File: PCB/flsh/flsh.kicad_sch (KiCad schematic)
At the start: 10 parts, among them U1 0.18Ω, U2 0.18Ω, U3 0.18Ω, U4 0.18Ω, U5 0.18Ω

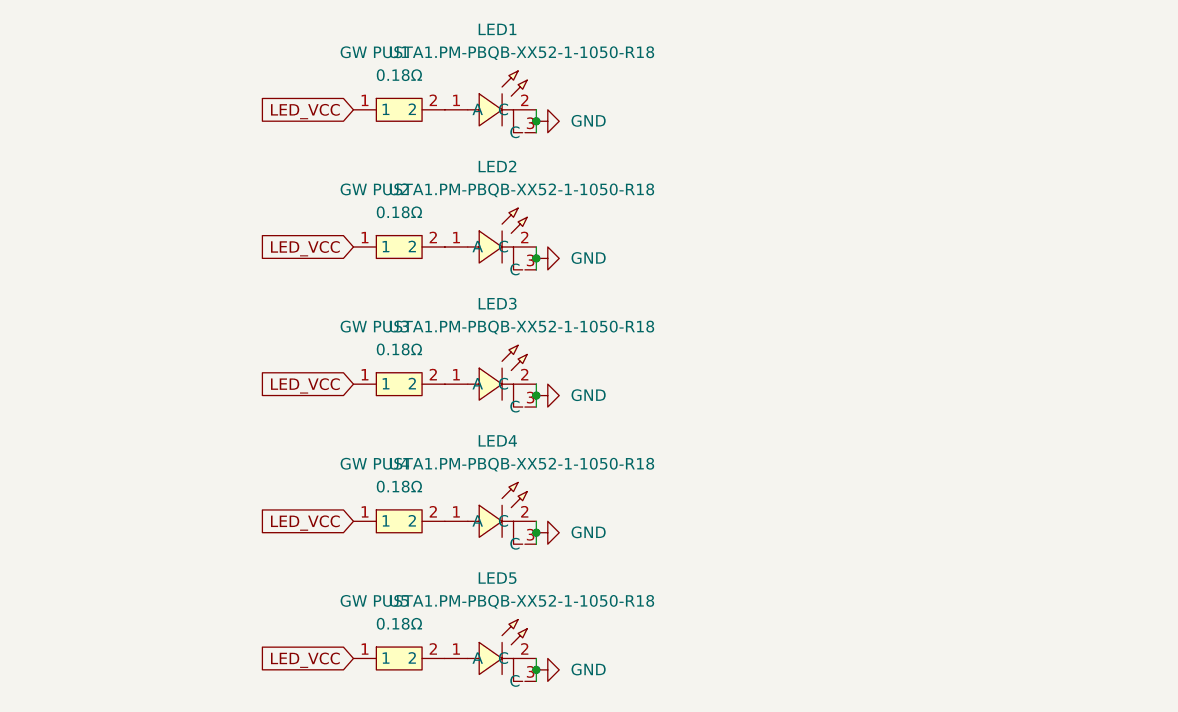
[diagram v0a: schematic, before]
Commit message: flsh!!
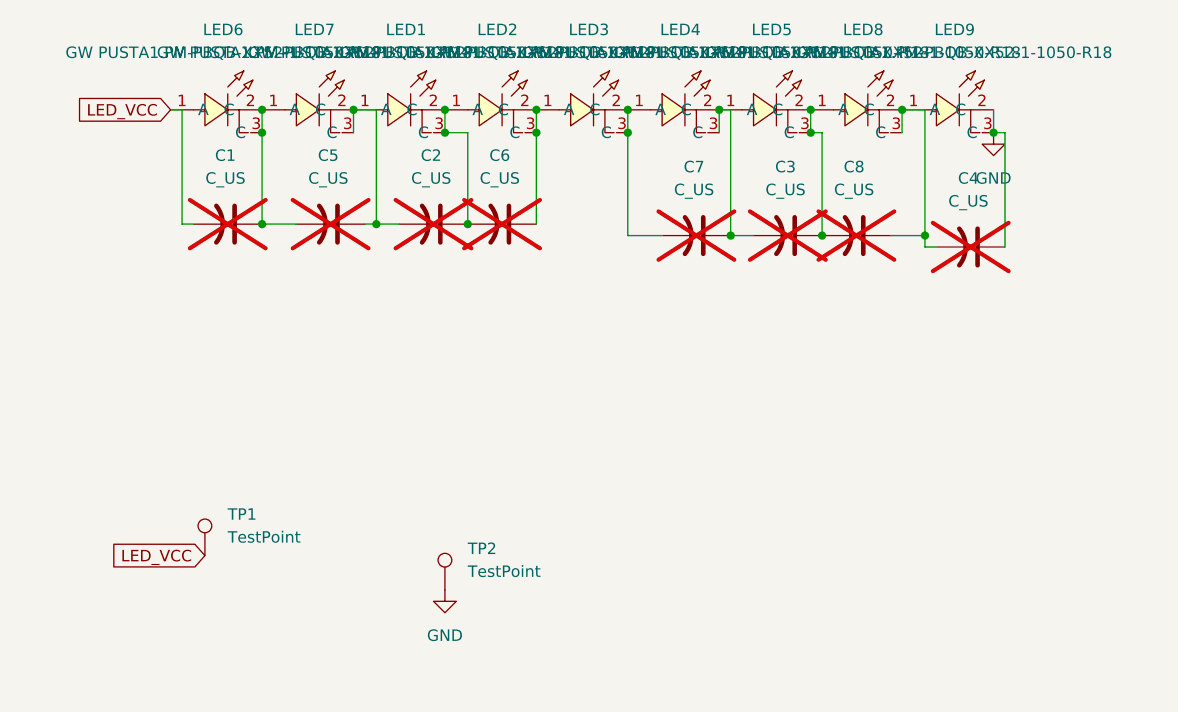
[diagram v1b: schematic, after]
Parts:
- removed U1, U2, U3, U4, U5: 0.18Ω, easyeda2kicad:R1206, symbol lcsc:HOLRT1206-1W-180MR-1%
- added C1, C2, C3, C4, C5, C6, C7, C8: C_US, Capacitor_SMD:C_1206_3216Metric, symbol Device:C_US
- added LED6, LED7, LED8, LED9: GW PUSTA1.PM-PBQB-XX52-1-1050-R18, easyeda2kicad:LED-SMD_3P-L3.7-W3.7_GW-PUSTA1.PM-NAPD-XX510-1-1050-R18, symbol lcsc:GWPUSTA1.PM-PBQB-XX52-1-1050-R18
- added TP1, TP2: TestPoint, TestPoint:TestPoint_Pad_D1.0mm, symbol Connector:TestPoint
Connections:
- net GND: now also C4.1, LED9.2 (C), LED9.3 (C), TP2.1; no longer LED1.2 (C), LED1.3 (C), LED2.2 (C), LED2.3 (C), LED3.2 (C), LED3.3 (C), LED4.2 (C), LED4.3 (C), LED5.2 (C), LED5.3 (C)
- net LED_VCC: now also C1.2, LED6.1 (A), TP1.1
- net at LED5.1 (A): now also LED4.2 (C), LED4.3 (C), C3.2, C7.1
- net at LED2.1 (A): now also LED1.2 (C), LED1.3 (C), C2.1, C6.2
- net at LED1.1 (A): now also C2.2, C5.1, LED7.2 (C), LED7.3 (C)
- net at LED3.1 (A): now also LED2.2 (C), LED2.3 (C), C6.1
- net at LED4.1 (A): now also LED3.2 (C), LED3.3 (C), C7.2
- new net: C1.1, C5.2, LED6.2 (C), LED6.3 (C), LED7.1 (A)
- new net: C3.1, C8.2, LED5.2 (C), LED5.3 (C), LED8.1 (A)
- new net: C4.2, C8.1, LED8.2 (C), LED8.3 (C), LED9.1 (A)
